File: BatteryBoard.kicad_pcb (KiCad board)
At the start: 4 copper layers, 13.2 x 10.4 mm, 18 parts, among them J1 Conn_01x05_Pin, J2 Conn_01x05_Pin, U1 BQ25619ERTWR

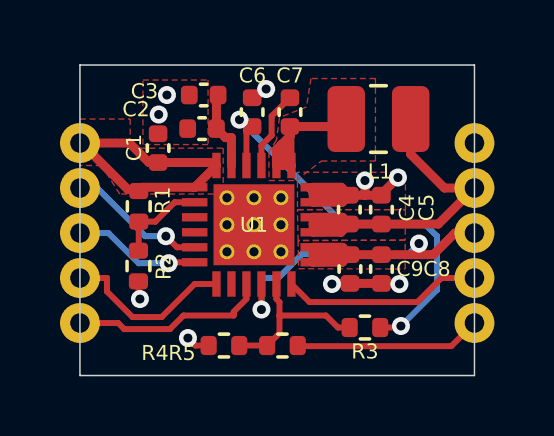
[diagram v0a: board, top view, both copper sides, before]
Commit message: Teardropped Vias
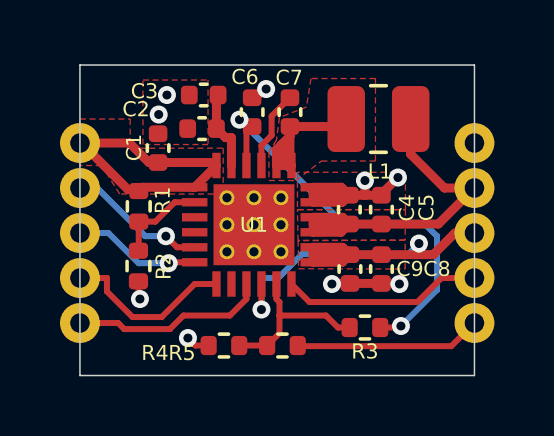
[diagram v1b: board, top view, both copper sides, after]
